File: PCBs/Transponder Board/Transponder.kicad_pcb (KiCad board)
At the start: 2 copper layers, 64 x 87.4 mm, 27 parts, among them J1 Conn_01x02, J2 Conn_01x02, J3 Conn_01x02, J4 Conn_01x02, J5 Conn_01x02, J6 Conn_01x09, U1 R-78E3.3-0.5, U2 MicroSDBreakout, U3 XBee-S2C, U4 PI4ULS5V201TAEX

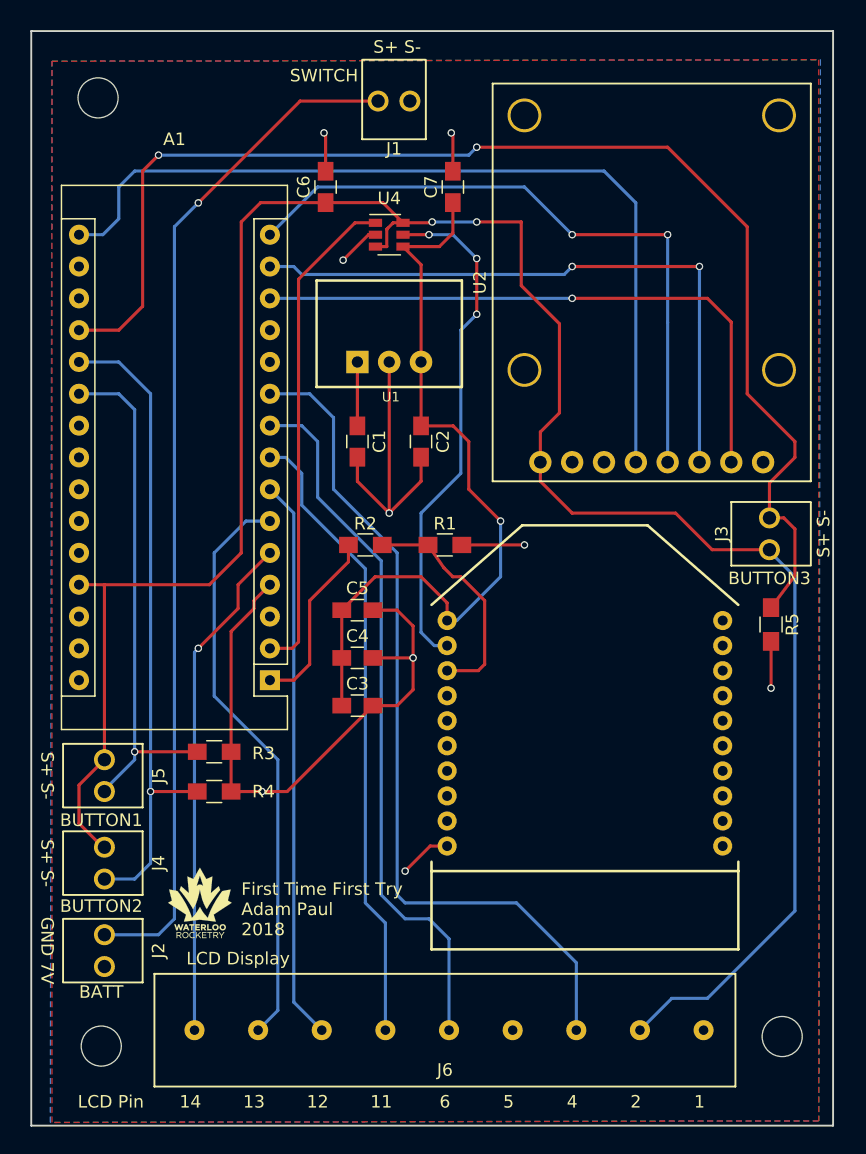
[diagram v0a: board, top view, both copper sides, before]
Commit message: transponder changes as per Alexs review
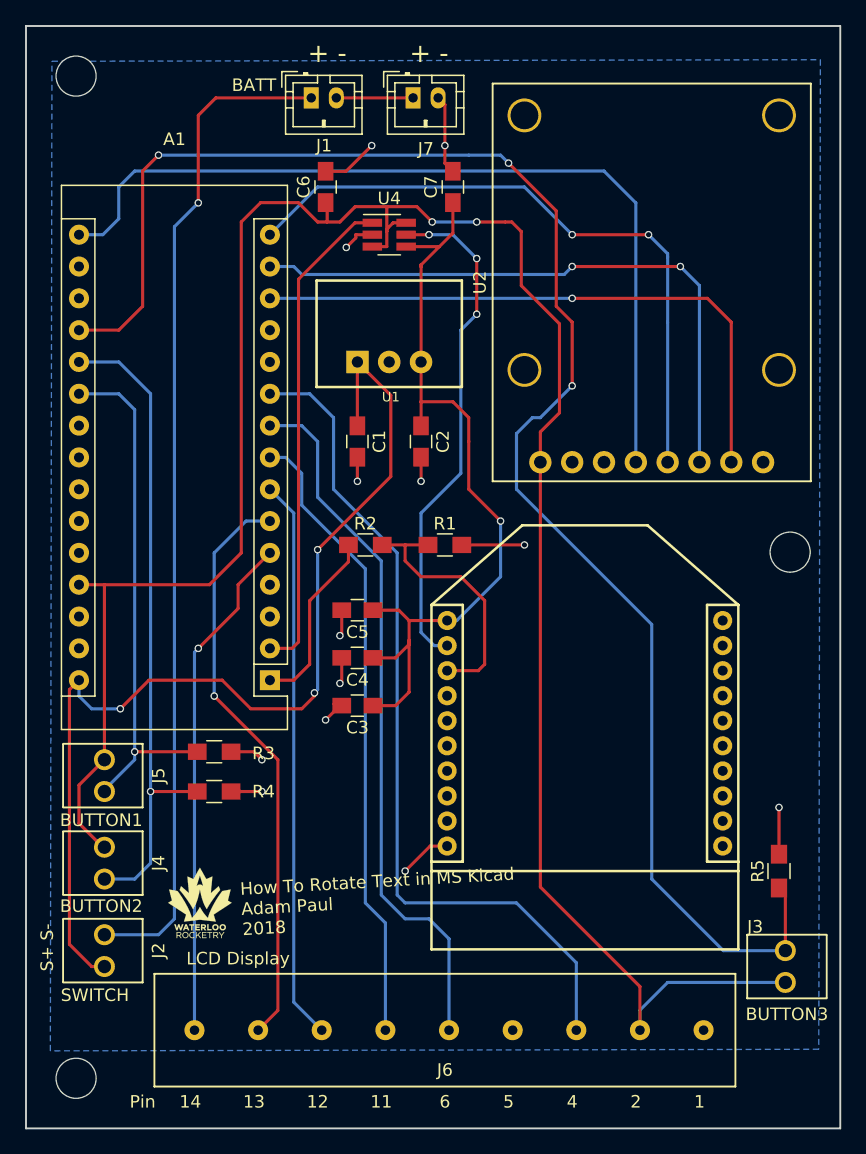
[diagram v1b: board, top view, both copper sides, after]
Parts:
- added J7: Conn_01x02, Connectors_JST:JST_PH_B2B-PH-K_02x2.00mm_Straight, F.Cu at (88.9, 62.7)
- J1: footprint molex:molex_kk_22-23-2021 -> Connectors_JST:JST_PH_B2B-PH-K_02x2.00mm_Straight
- U4: footprint sot:SOT-23-6 -> TO_SOT_Packages_SMD:SOT-23-6_Handsoldering
- moved REF** 38.7 mm to (119.0, 99.0)
- moved J3 34.6 mm to (115.6, 132.1)
- moved R5 19.7 mm to (118.1, 124.5), turned to 90 degrees
- moved J1 7.38 mm to (80.8, 62.7)
- moved REF** 3.26 mm to (62.0, 141.0)
- moved REF** 2.47 mm to (62.0, 61.0)
- turned C3 to 180 degrees
- turned C4 to 180 degrees
- turned C5 to 180 degrees
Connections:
- J1 pad 2: GND -> Net-(J1-Pad2)
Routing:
- net 7.4V: track 5.10 -> 83.1 mm, vias 0 -> 3
- net GND: track 93.4 -> 43.8 mm, vias 9 -> 13
- net D2: track 103.3 -> 130.8 mm, vias 2 -> 3
- net Net-(J1-Pad2): track 0.00 -> 6.13 mm
- net Net-(R1-Pad1): track 18.5 -> 20.9 mm
- net Net-(J1-Pad1): track 81.8 -> 80.6 mm
- net 3.3V: track 64.2 -> 65.3 mm
- net 5V: track 179.8 -> 178.6 mm
- net MOSI: track 50.4 -> 49.5 mm
- net MISO: track 53.1 -> 52.2 mm
- net LCD_D6: vias 0 -> 1
- removed copper zone on F.Cu, net 7.4V
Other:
- board size 64 x 87.4 mm -> 65 x 88 mm
- rule pad_to_mask_clearance: 0.2 -> 0.002
- board text added: "+ -"
- board text added: "How To Rotate Text in MS Kicad Adam Paul 2018"
- board text added: "Pin"
- board text removed: "First Time First Try Adam Paul 2018"
- board text removed: "GND 7V"
- board text removed: "LCD Pin"

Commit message: fixed outstanding changes on instr and transponder board
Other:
- rule pad_to_mask_clearance: 0.002 -> 0.0508
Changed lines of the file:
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@@
     (links 60)
     (no_connects 0)
-    (area 57.924999 56.924999 123.075001 145.075001)
+    (area 51.021143 55.825 128.557143 146.275)
     (thickness 1.6)
     (drawings 24)
@@
     (pad_size 1.524 1.524)
     (pad_drill 0.762)
-    (pad_to_mask_clearance 0.002)
+    (pad_to_mask_clearance 0.0508)
     (aux_axis_origin 0 0)
     (visible_elements 7FFFFF7F)
